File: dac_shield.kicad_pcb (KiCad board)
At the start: 2 copper layers, 68.6 x 53.3 mm, 33 parts, among them P1 CONN_2, P2 CONN_2, P3 CONN_2, T1 VrefTest, U1 MCP4921, U2 TCA0372, U3 LM741

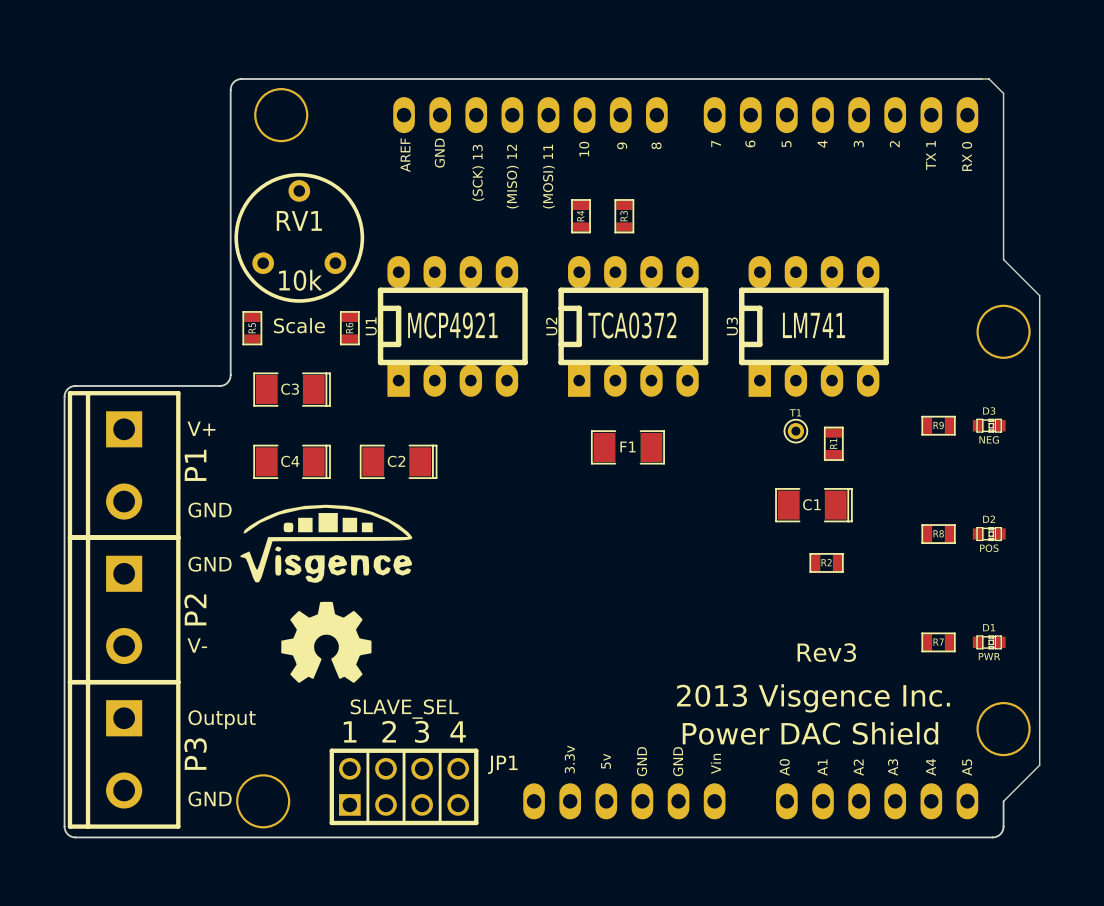
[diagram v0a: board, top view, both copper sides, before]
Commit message: First route and fill
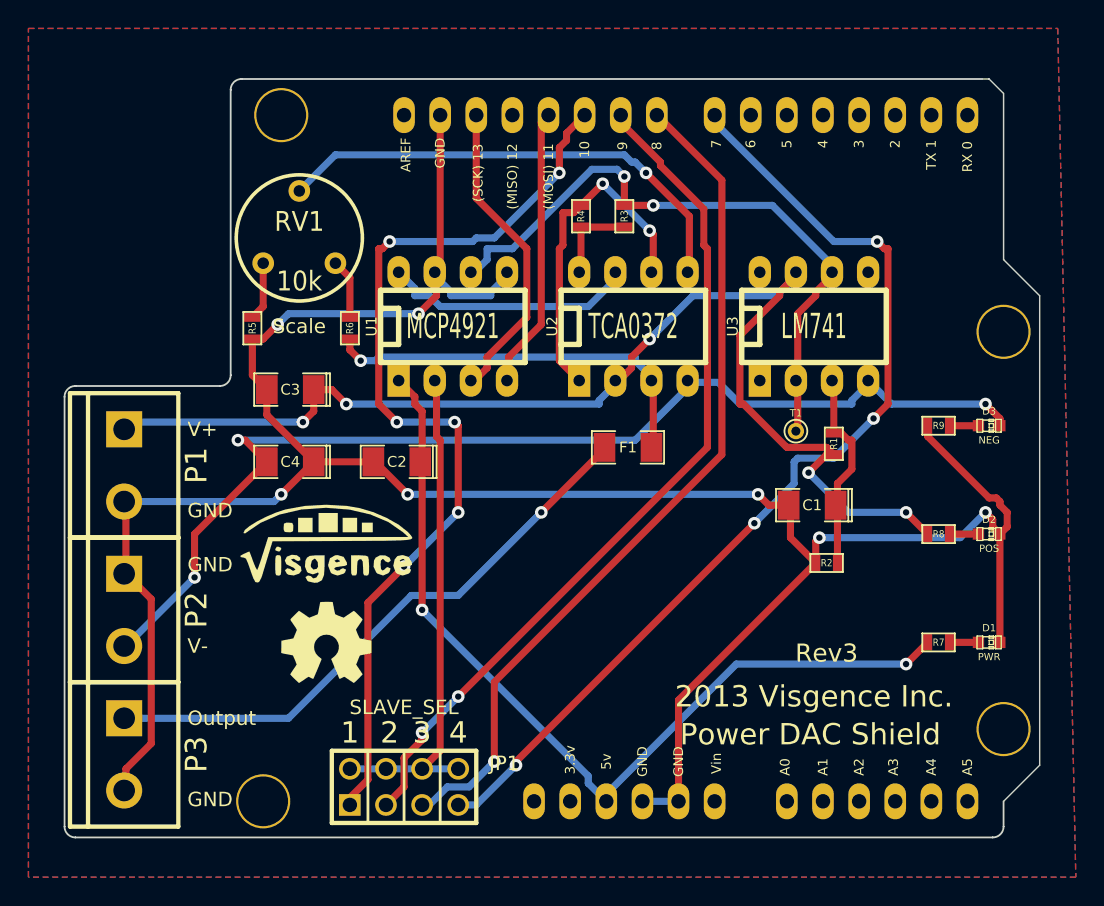
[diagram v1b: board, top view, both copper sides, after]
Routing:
- net GND: track 0.00 -> 178.9 mm, vias 0 -> 7
- net VDD: track 0.00 -> 86.2 mm, vias 0 -> 5
- net VSS: track 0.00 -> 78.8 mm, vias 0 -> 3
- net N-0000034: track 0.00 -> 70.3 mm, vias 0 -> 4
- net N-0000036: track 0.00 -> 66.7 mm, vias 0 -> 6
- net +5V: track 0.00 -> 63.4 mm, vias 0 -> 2
- net N-0000033: track 0.00 -> 60.4 mm, vias 0 -> 2
- net N-0000035: track 0.00 -> 60.3 mm, vias 0 -> 1
- net VREF: track 0.00 -> 46.6 mm, vias 0 -> 2
- net N-000009: track 0.00 -> 41.9 mm, vias 0 -> 1
- net N-0000037: track 0.00 -> 35.6 mm
- net N-0000044: track 0.00 -> 34.5 mm, vias 0 -> 1
- net N-000007: track 0.00 -> 28.6 mm, vias 0 -> 1
- net N-0000043: track 0.00 -> 24.1 mm, vias 0 -> 2
- net CLK: track 0.00 -> 21.9 mm
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- added copper zone on B.Cu, net GND
- added copper zone on F.Cu, net GND
